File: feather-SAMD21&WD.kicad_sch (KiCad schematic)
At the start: 42 parts, among them J1 left_header, J10 reset_enable, J2 Batt_header, J3 right_header, J5 16P_USB_C, J6 JumperSET0, J8 JumperSET1, J9 JumperSET2, SW3 SW_Push, U1 ATSAMD21G18A-M, U2 AMS1117-3.3, U3 MAX6369, U5 USBLC6-2SC6

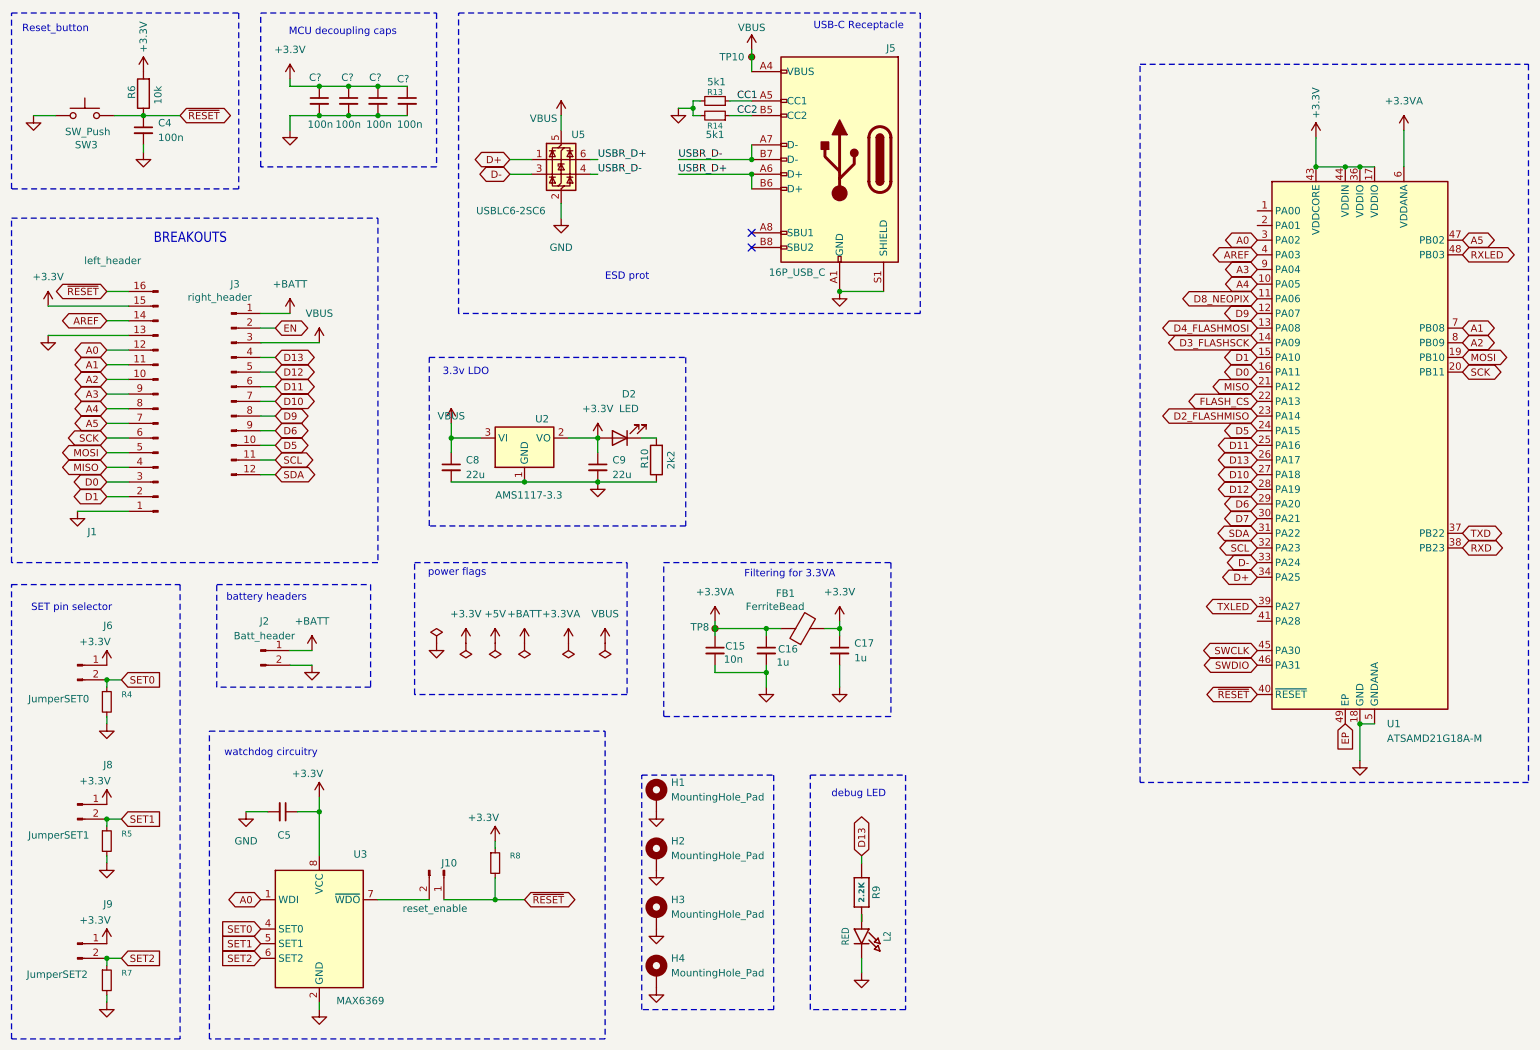
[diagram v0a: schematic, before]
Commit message: minor changes
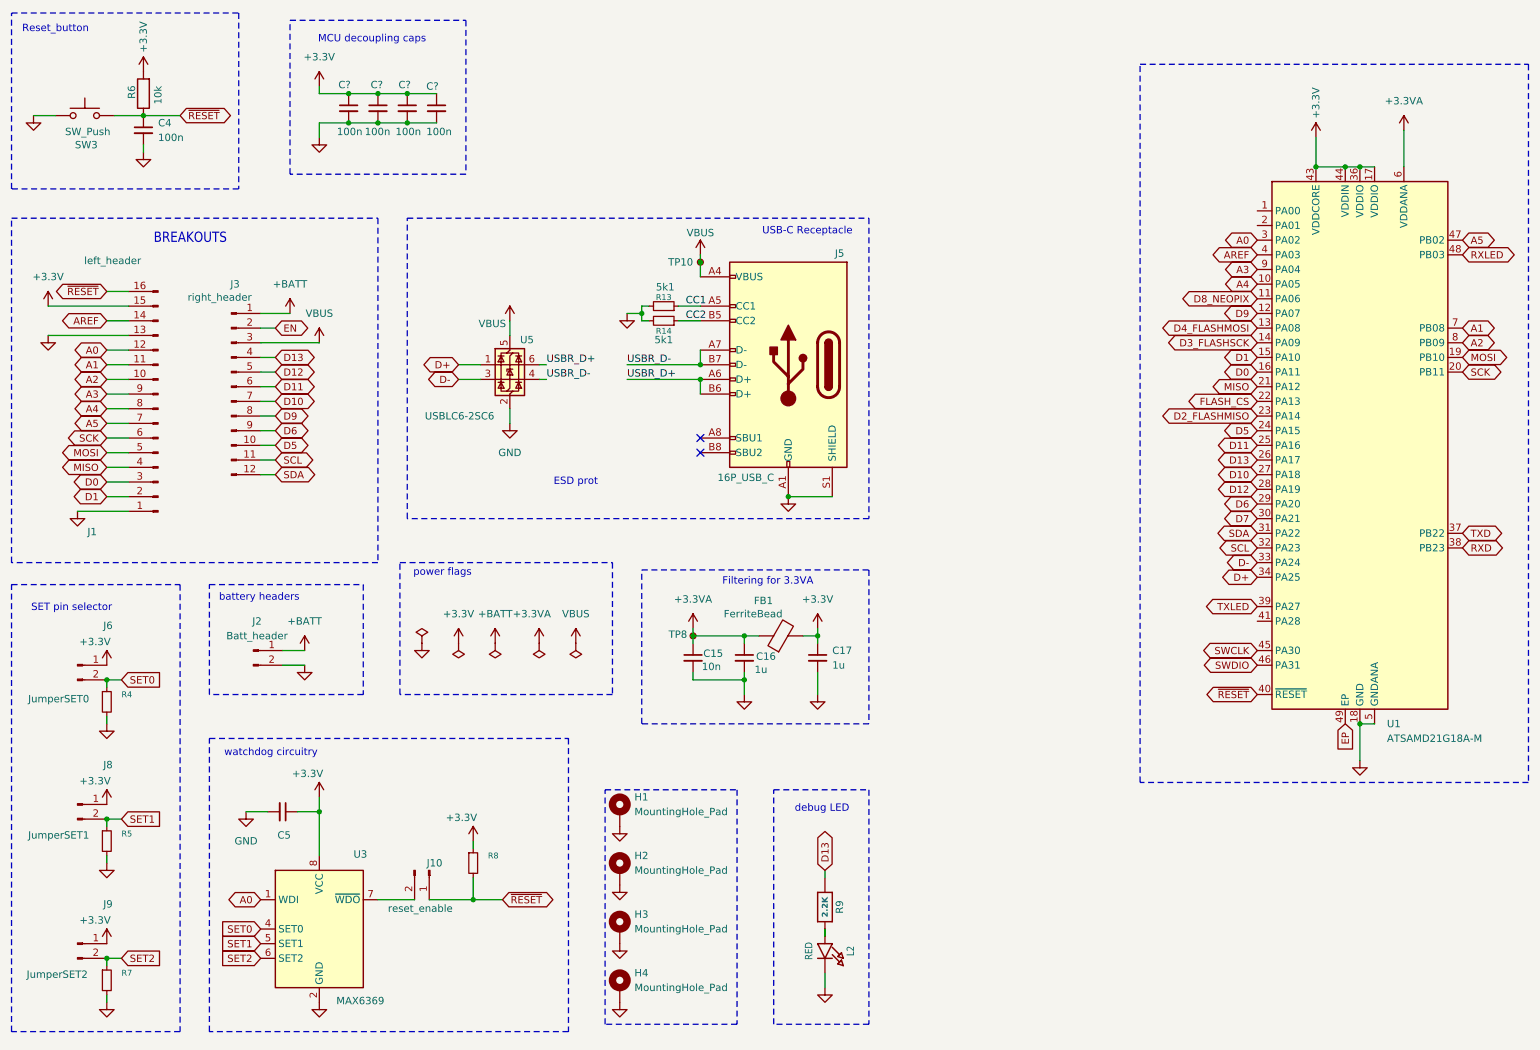
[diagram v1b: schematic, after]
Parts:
- removed C8, C9: 22u, Capacitor_SMD:C_0805_2012Metric_Pad1.18x1.45mm_HandSolder, symbol Device:C_Small
- removed D2: LED, LED_SMD:LED_0805_2012Metric_Pad1.15x1.40mm_HandSolder, symbol Device:LED
- removed R10: 2k2, Resistor_SMD:R_0805_2012Metric_Pad1.20x1.40mm_HandSolder, symbol Device:R
- removed U2: AMS1117-3.3, Package_TO_SOT_SMD:SOT-223-3_TabPin2, symbol Regulator_Linear:AMS1117-3.3
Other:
- note removed: "3.3v LDO"
- moved on the sheet: C15, C16, C17, C?, FB1, H1, H2, H3, H4, J10, J2, J5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
